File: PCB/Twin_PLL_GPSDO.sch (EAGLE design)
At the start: 140 parts, among them IC1 ADP151WAUJZ-1.8-R7, IC2 ADP151WAUJZ-1.8-R7, IC3 MCP4725A0T-E_CH, IC4 LT1963AEQ-2.5#PBF, T1 BC847, U2 ADF4351BCPZ, U3 ADF4351BCPZ

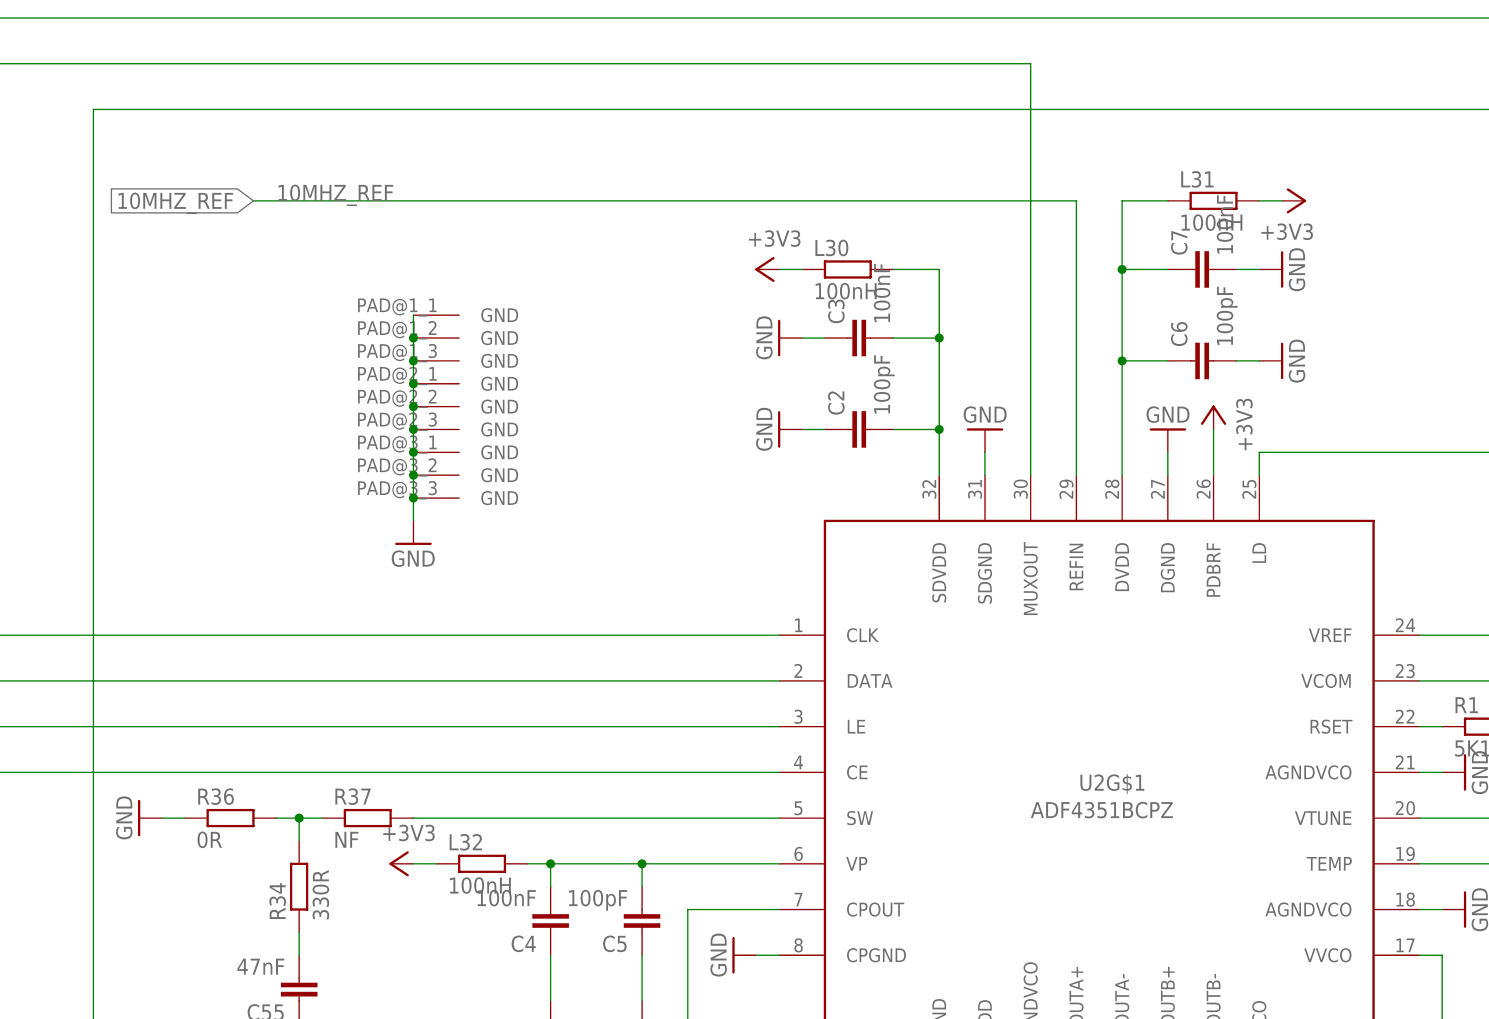
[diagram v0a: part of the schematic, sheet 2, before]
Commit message: initial corrections to producion PCB
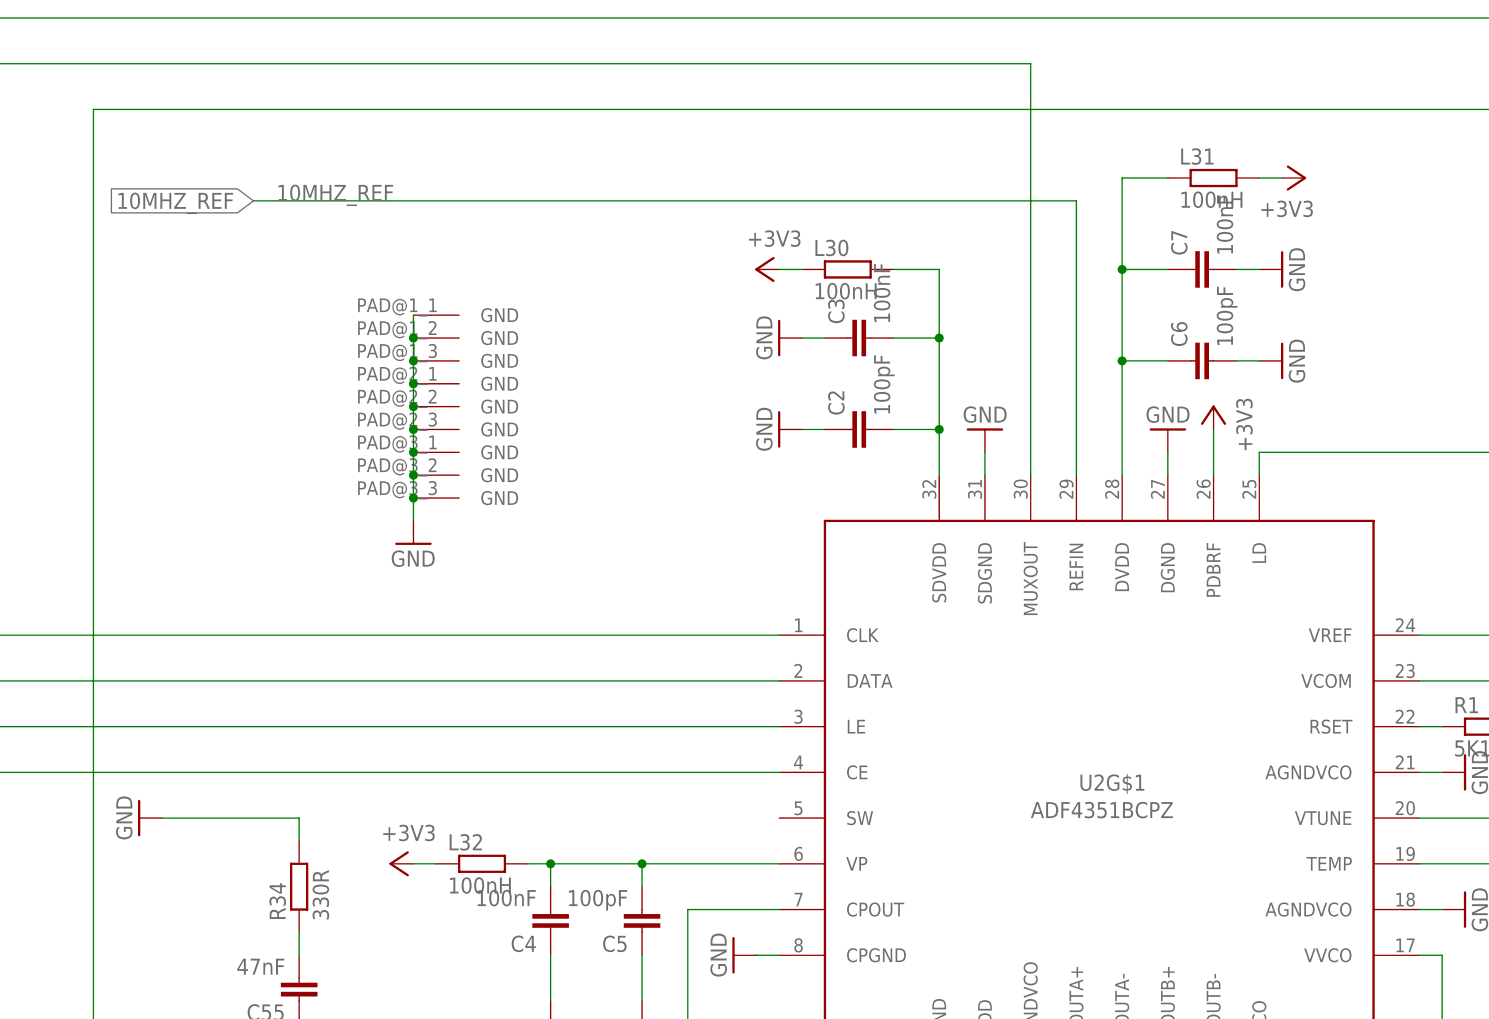
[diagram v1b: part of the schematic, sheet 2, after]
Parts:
- removed R36, R7: 0R, rcl:R-EU_R0603
- removed R37, R8: NF, rcl:R-EU_R0603
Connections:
- removed net N$15: R5.2, R7.2, R8.1
- removed net N$16: R8.2, U3G$1.SW
- removed net N$49: R34.2, R36.2, R37.1
- removed net N$50: R37.2, U2G$1.SW
- net GND: now also R34.2, R5.2; no longer R36.1, R7.1
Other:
- moved on the sheet: L31
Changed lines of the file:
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@@
 <part name="R35" library="resistor" deviceset="R-EU_" device="R0603" value="680R"/>
 <part name="C56" library="rcl" deviceset="C-EU" device="C0603" value="1N5"/>
-<part name="R36" library="rcl" deviceset="R-EU_" device="R0603" value="0R"/>
-<part name="R37" library="rcl" deviceset="R-EU_" device="R0603" value="NF"/>
 <part name="GND50" library="supply1" deviceset="GND" device=""/>
 <part name="GND51" library="supply1" deviceset="GND" device=""/>
@@
 <part name="R6" library="resistor" deviceset="R-EU_" device="R0603" value="680R"/>
 <part name="C68" library="rcl" deviceset="C-EU" device="C0603" value="1N5"/>
-<part name="R7" library="rcl" deviceset="R-EU_" device="R0603" value="0R"/>
-<part name="R8" library="rcl" deviceset="R-EU_" device="R0603" value="NF"/>
 <part name="GND62" library="supply1" deviceset="GND" device=""/>
 <part name="GND63" library="supply1" deviceset="GND" device=""/>
@@
 <instance part="GND41" gate="1" x="266.7" y="81.28"/>
 <instance part="+3V4" gate="G$1" x="165.1" y="223.52" rot="MR270"/>
-<instance part="+3V5" gate="G$1" x="226.06" y="231.14" rot="MR90"/>
+<instance part="+3V5" gate="G$1" x="226.06" y="233.68" rot="MR90"/>
 <instance part="+3V6" gate="G$1" x="190.5" y="93.98" rot="MR180"/>
 <instance part="+3V7" gate="G$1" x="124.46" y="157.48" rot="MR270"/>
@@
 <instance part="R35" gate="G$1" x="101.6" y="134.62"/>
 <instance part="C56" gate="G$1" x="91.44" y="124.46" rot="R180"/>
-<instance part="R36" gate="G$1" x="106.68" y="162.56"/>
-<instance part="R37" gate="G$1" x="121.92" y="162.56"/>
 <instance part="GND50" gate="1" x="91.44" y="116.84"/>
 <instance part="GND51" gate="1" x="114.3" y="116.84"/>
@@
 <instance part="L32" gate="G$1" x="134.62" y="157.48"/>
 <instance part="L30" gate="G$1" x="175.26" y="223.52"/>
-<instance part="L31" gate="G$1" x="215.9" y="231.14"/>
+<instance part="L31" gate="G$1" x="215.9" y="233.68"/>
 <instance part="L27" gate="G$1" x="248.92" y="127"/>
 <instance part="U$7" gate="CCSA" x="302.26" y="0"/>
@@
 <pinref part="GND41" gate="1" pin="GND"/>
 <pinref part="C51" gate="G$1" pin="1"/>
-</segment>
-<segment>
-<wire x1="101.6" y1="162.56" x2="99.06" y2="162.56" width="0.1524" layer="91"/>
-<pinref part="R36" gate="G$1" pin="1"/>
-<pinref part="GND52" gate="1" pin="GND"/>
 </segment>
 <segment>
@@
 <label x="281.94" y="60.96" size="1.778" layer="95" rot="R180"/>
 </segment>
+<segment>
+<pinref part="GND52" gate="1" pin="GND"/>
+<pinref part="R34" gate="G$1" pin="2"/>
+<wire x1="99.06" y1="162.56" x2="114.3" y2="162.56" width="0.1524" layer="91"/>
+<wire x1="114.3" y1="162.56" x2="114.3" y2="160.02" width="0.1524" layer="91"/>
+</segment>
 </net>
 <net name="+3V3_ADF1" class="0">
@@
 <pinref part="+3V5" gate="G$1" pin="+3V3"/>
 <pinref part="L31" gate="G$1" pin="2"/>
-<wire x1="223.52" y1="231.14" x2="220.98" y2="231.14" width="0.1524" layer="91"/>
+<wire x1="223.52" y1="233.68" x2="220.98" y2="233.68" width="0.1524" layer="91"/>
 </segment>
 </net>
@@
 </segment>
 </net>
-<net name="N$49" class="0">
-<segment>
-<wire x1="114.3" y1="160.02" x2="114.3" y2="162.56" width="0.1524" layer="91"/>
-<wire x1="114.3" y1="162.56" x2="111.76" y2="162.56" width="0.1524" layer="91"/>
-<wire x1="114.3" y1="162.56" x2="116.84" y2="162.56" width="0.1524" layer="91"/>
-<junction x="114.3" y="162.56"/>
-<pinref part="R34" gate="G$1" pin="2"/>
-<pinref part="R36" gate="G$1" pin="2"/>
-<pinref part="R37" gate="G$1" pin="1"/>
-</segment>
-</net>
-<net name="N$50" class="0">
-<segment>
-<wire x1="127" y1="162.56" x2="167.64" y2="162.56" width="0.1524" layer="91"/>
-<pinref part="R37" gate="G$1" pin="2"/>
-<pinref part="U2" gate="G$1" pin="SW"/>
-</segment>
-</net>
 <net name="ADF1_LD" class="0">
 <segment>
@@
 <pinref part="C7" gate="G$1" pin="1"/>
 <pinref part="L31" gate="G$1" pin="1"/>
-<wire x1="210.82" y1="231.14" x2="205.74" y2="231.14" width="0.1524" layer="91"/>
-<wire x1="205.74" y1="231.14" x2="205.74" y2="223.52" width="0.1524" layer="91"/>
+<wire x1="210.82" y1="233.68" x2="205.74" y2="233.68" width="0.1524" layer="91"/>
+<wire x1="205.74" y1="233.68" x2="205.74" y2="223.52" width="0.1524" layer="91"/>
 <junction x="205.74" y="223.52"/>
 </segment>
@@
 <instance part="R6" gate="G$1" x="101.6" y="134.62"/>
 <instance part="C68" gate="G$1" x="91.44" y="124.46" rot="R180"/>
-<instance part="R7" gate="G$1" x="106.68" y="162.56"/>
-<instance part="R8" gate="G$1" x="121.92" y="162.56"/>
 <instance part="GND62" gate="1" x="91.44" y="116.84"/>
 <instance part="GND63" gate="1" x="114.3" y="116.84"/>
@@
 </segment>
 </net>
-<net name="N$15" class="0">
-<segment>
-<wire x1="114.3" y1="160.02" x2="114.3" y2="162.56" width="0.1524" layer="91"/>
-<wire x1="114.3" y1="162.56" x2="111.76" y2="162.56" width="0.1524" layer="91"/>
-<wire x1="114.3" y1="162.56" x2="116.84" y2="162.56" width="0.1524" layer="91"/>
-<junction x="114.3" y="162.56"/>
-<pinref part="R5" gate="G$1" pin="2"/>
-<pinref part="R7" gate="G$1" pin="2"/>
-<pinref part="R8" gate="G$1" pin="1"/>
-</segment>
-</net>
-<net name="N$16" class="0">
-<segment>
-<wire x1="127" y1="162.56" x2="167.64" y2="162.56" width="0.1524" layer="91"/>
-<pinref part="R8" gate="G$1" pin="2"/>
-<pinref part="U3" gate="G$1" pin="SW"/>
-</segment>
-</net>
 <net name="ADF2_LD" class="0">
 <segment>
@@
 <pinref part="GND61" gate="1" pin="GND"/>
 <pinref part="C63" gate="G$1" pin="1"/>
-</segment>
-<segment>
-<wire x1="101.6" y1="162.56" x2="99.06" y2="162.56" width="0.1524" layer="91"/>
-<pinref part="R7" gate="G$1" pin="1"/>
-<pinref part="GND64" gate="1" pin="GND"/>
 </segment>
 <segment>
@@
 <wire x1="274.32" y1="60.96" x2="274.32" y2="71.12" width="0.1524" layer="91"/>
 </segment>
-</net>
+<segment>
+<pinref part="GND64" gate="1" pin="GND"/>
+<pinref part="R5" gate="G$1" pin="2"/>
+<wire x1="99.06" y1="162.56" x2="114.3" y2="162.56" width="0.1524" layer="91"/>
+<wire x1="114.3" y1="162.56" x2="114.3" y2="160.02" width="0.1524" layer="91"/>
+</segment>
+</net>
